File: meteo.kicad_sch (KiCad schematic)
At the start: 29 parts, among them J1 mlab I2C, J10 Eth, J11 I2C0, J12 I2C1, J13 I2C2, J14 I2C3, J15 UART, J16 UART pow, J17 5V jumper, J18 power control circuit, J2 SPI, J3 Analog, J4 Conn_02x19_Odd_Even, J5 Conn_02x18_Odd_Even, J6 I/O, J7 mlab_pow, J9 SD, U1 CD74HC4067M, U2 CD74HC4067M, U3 multiplex analog, U4 ADS1015IDGS, U5 PCF8575DBR

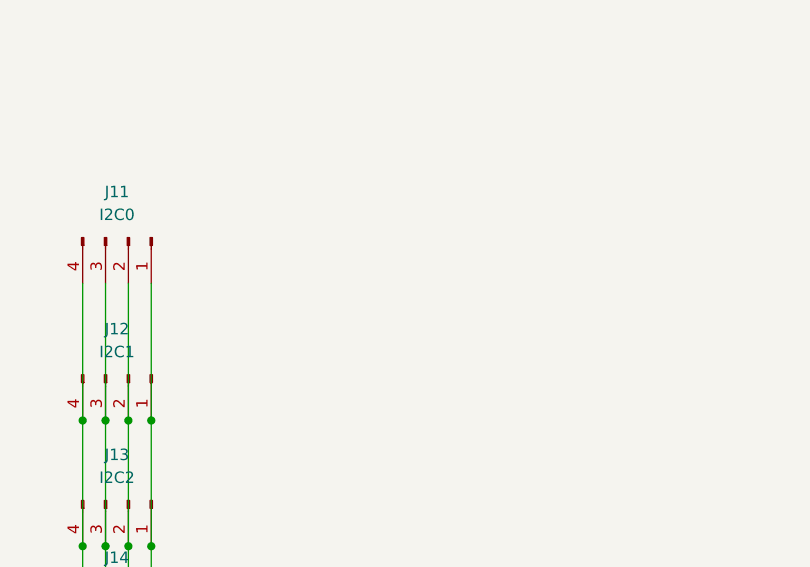
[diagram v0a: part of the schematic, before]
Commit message: Oprava děr
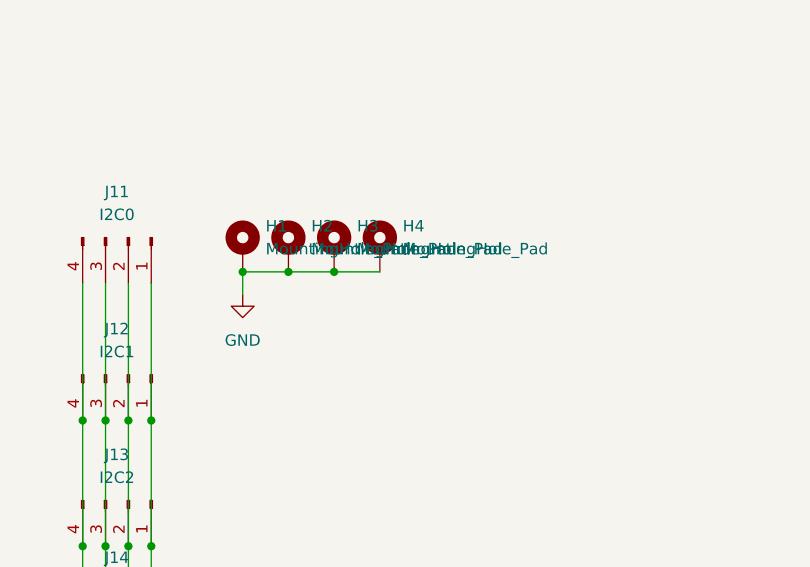
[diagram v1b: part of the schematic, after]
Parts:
- added H1, H2, H3, H4: MountingHole_Pad, MountingHole:MountingHole_3.2mm_M3_DIN965_Pad, symbol Mechanical:MountingHole_Pad
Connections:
- net GND: now also H1.1, H2.1, H3.1, H4.1
